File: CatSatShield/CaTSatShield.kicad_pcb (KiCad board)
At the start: 4 copper layers, 67.6 x 25 mm, 17 parts, among them J1 , J2 , J3 BME280, J4 CCS811

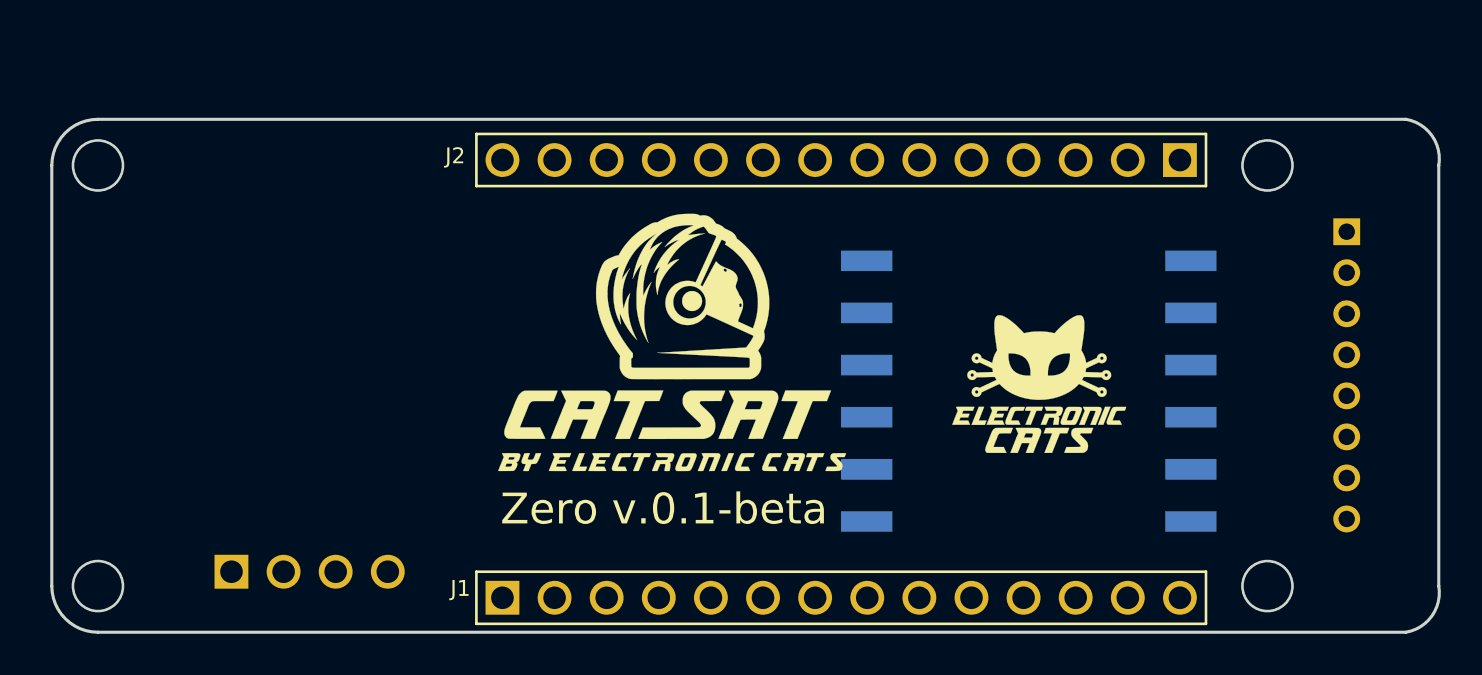
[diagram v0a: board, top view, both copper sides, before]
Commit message: Routeo
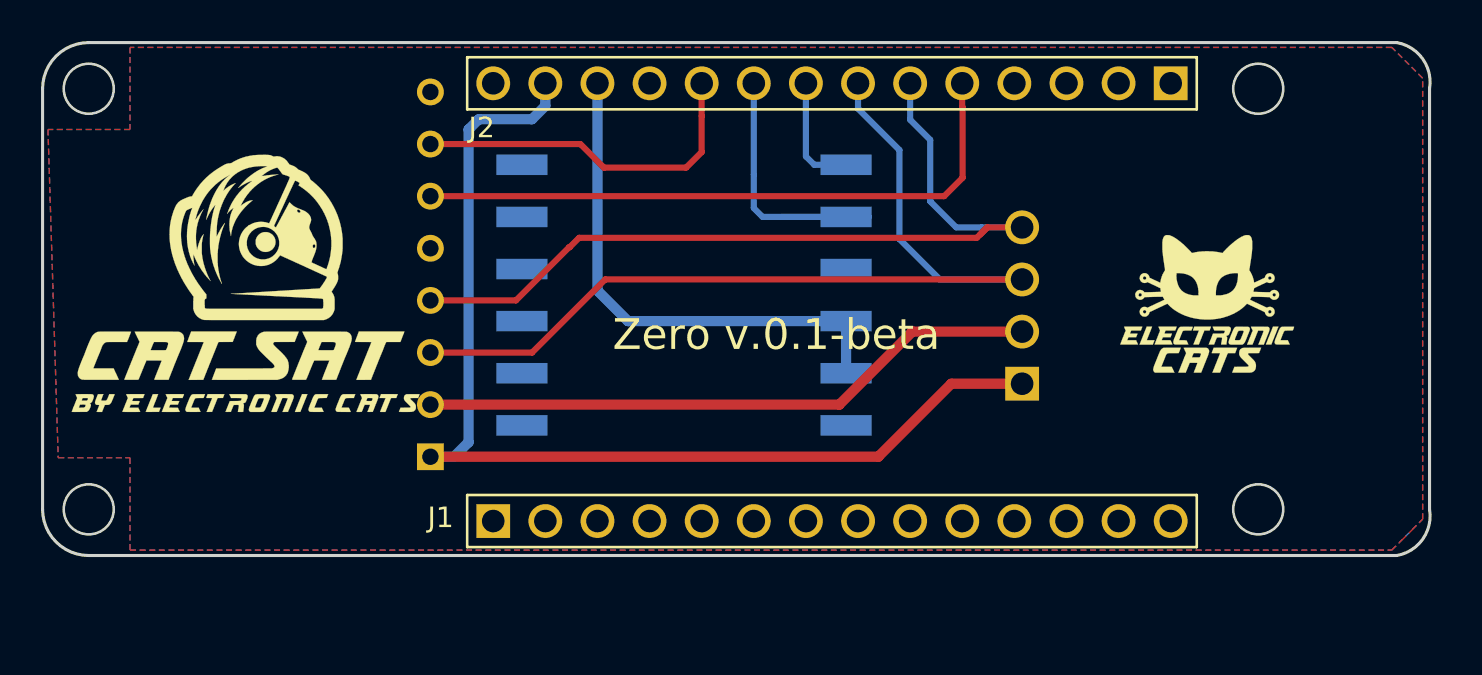
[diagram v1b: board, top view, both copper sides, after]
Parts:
- moved J4 44.9 mm to (133.1, 100.1), turned to 90 degrees
- moved J3 37.1 mm to (162.0, 101.6), turned to 90 degrees
- moved G*** 31.1 mm to (172.5, 100.0)
- moved G*** 21.0 mm to (124.5, 100.5)
- moved MODULE1 17.4 mm to (145.5, 100.2)
- moved G*** 9.07 mm to (171.0, 101.5)
- moved @HOLE0 3.77 mm to (116.5, 111.5)
- moved @HOLE1 3.77 mm to (116.5, 91.0)
- moved U$5 3.77 mm to (116.5, 111.5)
- moved U$6 3.77 mm to (116.5, 91.0)
- moved @HOLE2 3.77 mm to (173.5, 91.0)
- moved @HOLE3 3.77 mm to (173.5, 111.5)
- moved U$7 3.77 mm to (173.5, 91.0)
- moved U$8 3.77 mm to (173.5, 111.5)
- moved J1 3.77 mm to (152.7, 112.1)
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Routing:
- net VCC: track 0.00 -> 53.0 mm
- net /SCL: track 0.00 -> 45.5 mm
- net /SDA: track 0.00 -> 42.0 mm
- net /10-INTCCS: track 0.00 -> 30.9 mm
- net GND: track 0.00 -> 30.3 mm
- net +3V3: track 0.00 -> 25.4 mm
- net /RESET: track 0.00 -> 17.4 mm
- net /TX: track 0.00 -> 16.1 mm
- net /RX: track 0.00 -> 5.69 mm
- added copper zone on B.Cu, net GND
- added copper zone on F.Cu, net GND
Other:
- outline, holes or cut-outs redrawn
- net class Default: clearance 0.127 -> 0.2; trace_width 0.25 -> 0.3; via_dia 0.8 -> 1
- net class SOURCE added: clearance 0.2, trace_width 0.5, via_dia 1.2, via_drill 0.6
- rule trace_clearance: 0.127 -> 0.2
